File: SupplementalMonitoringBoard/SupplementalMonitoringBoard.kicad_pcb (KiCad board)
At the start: 2 copper layers, 53.5 x 77 mm, 47 parts, among them J1 PeripheralCANConnector, J2 PeripheralCANConnector, U1 OPA842xDBV, U2 OPA842xDBV, U3 INA180B1, U4 PAMC131M03QDFMRQ1, U5 PeripheralSOM

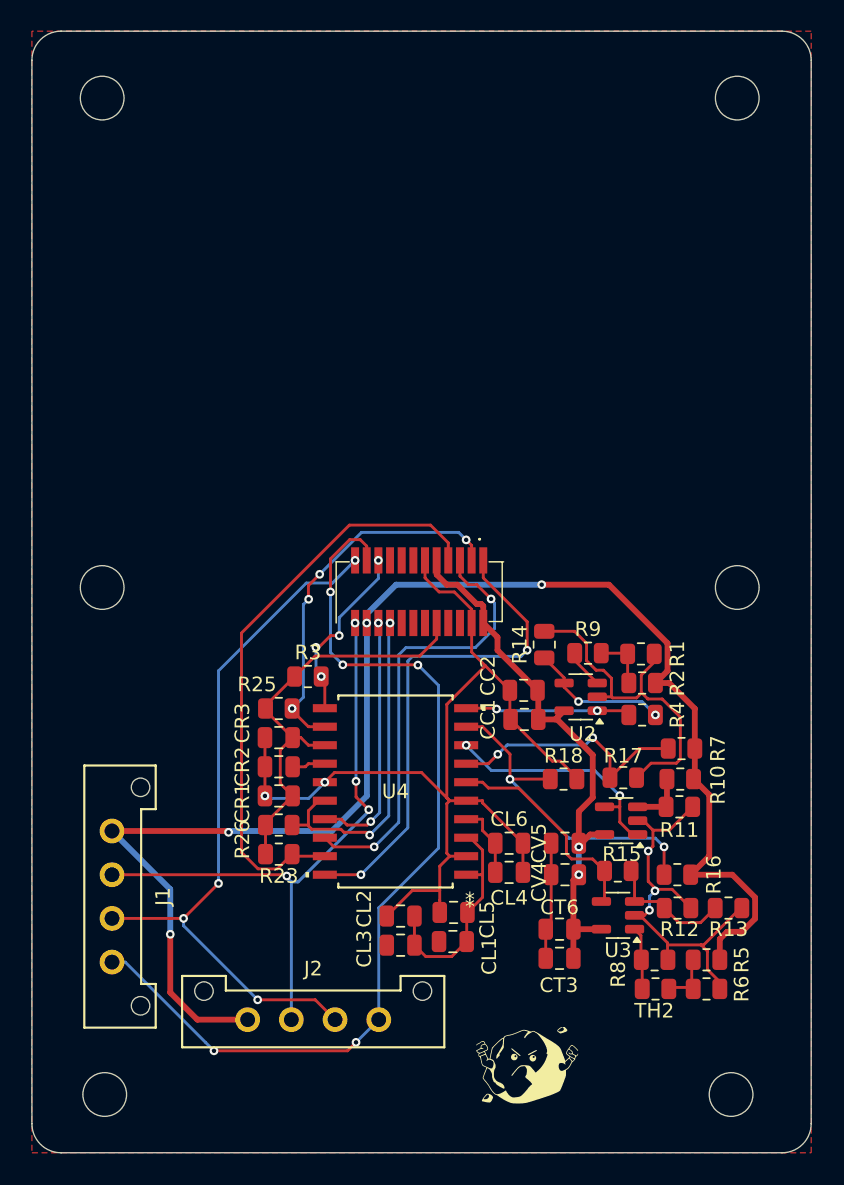
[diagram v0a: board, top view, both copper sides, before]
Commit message: Supplemental MOnitoring Board
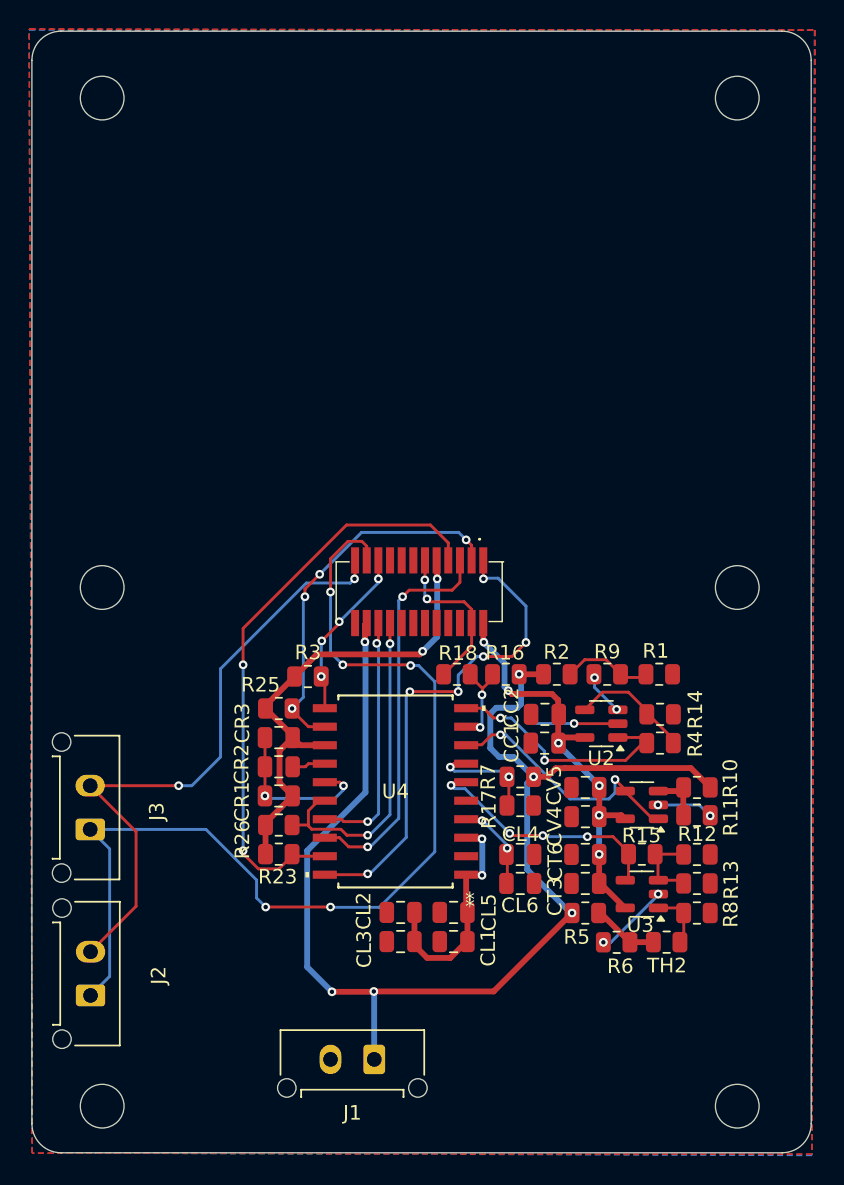
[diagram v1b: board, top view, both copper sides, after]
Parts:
- removed the ? at (124.5, 129.0)
- removed the ? at (167.5, 129.0)
- removed G***: LOGO, LOGO
- added ?: , , F.Cu at (167.9, 129.8)
- added ?: , , F.Cu at (124.3, 129.8)
- added J3: CANconn2, Connector_Molex:Molex_Micro-Fit_3.0_43650-0215_1x02_P3.00mm_Vertical, F.Cu at (123.5, 110.8)
- CC1, CT3, CV5: value .1uF -> 1nF
- CL2, CL5, CL6, CR1: value 1nF -> .1uF
- J1: value PeripheralCANConnector -> CarPowerConnector; footprint UTSVT_Connectors:Molex_MicroFit3.0_1x4xP3.00mm_PolarizingPeg_Vertical -> Connector_Molex:Molex_Micro-Fit_3.0_43650-0215_1x02_P3.00mm_Vertical
- J2: value PeripheralCANConnector -> CANconn; footprint UTSVT_Connectors:Molex_MicroFit3.0_1x4xP3.00mm_PolarizingPeg_Vertical -> Connector_Molex:Molex_Micro-Fit_3.0_43650-0215_1x02_P3.00mm_Vertical
- R14: value 150K -> 150k
- R2: value 50K -> 50k
- R4: value 10K -> 10k
- R7: value 30K -> 30k
- TH2: value 500 -> 500.
- moved J1 23.9 mm to (143.0, 126.6), turned to 180 degrees
- moved R16 18.1 mm to (152.0, 100.2)
- moved R7 11.2 mm to (153.0, 107.2)
- moved J2 10.9 mm to (123.5, 122.2), turned to 90 degrees
- moved R18 10.3 mm to (148.7, 100.2), turned to 180 degrees
- moved R14 9.28 mm to (162.6, 102.9), turned to 180 degrees
- moved R5 8.92 mm to (157.5, 116.5), turned to 180 degrees
- moved R17 7.32 mm to (153.0, 109.2)
- moved R6 6.95 mm to (159.6, 118.5), turned to 180 degrees
- moved R2 5.89 mm to (155.5, 100.2), turned to 180 degrees
- moved CT3 5.44 mm to (157.5, 114.5)
- moved CT6 5.43 mm to (157.5, 112.5)
- moved R8 4.33 mm to (165.2, 116.5)
- moved CV4 4.22 mm to (157.5, 109.9)
- moved CV5 4.08 mm to (157.5, 107.9)
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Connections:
- J1 pad 1: +BATT -> +12V
- J1 pad 2: GNDPWR -> GND
- J2 pad 1: +BATT -> /CAN_L
- J2 pad 2: GNDPWR -> /CAN_H
- R10 pad 2: +BATT -> +12V
- R16 pad 2: +BATT -> +12V
- R2 pad 2: +BATT -> +12V
- R5 pad 2: +BATT -> +12V
- R7 pad 2: +BATT -> +12V
- U5 pad 10: /DVDD -> unconnected-(U5-VDDA(3.3V)-Pad10)
- U5 pad 22: +BATT -> +12V
- U5 pad 9: +3.3V -> /DVDD
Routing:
- net +BATT: track 102.8 -> 0.00 mm, vias 4 -> 0
- net GND: track 131.7 -> 38.1 mm, vias 5 -> 9
- net +12V: track 0.00 -> 87.0 mm, vias 0 -> 6
- net GNDPWR: track 42.8 -> 0.00 mm, vias 4 -> 0
- net /AINOP: track 22.8 -> 5.97 mm
- net /AIN12N: track 17.5 -> 7.46 mm
- net +3.3V: track 38.4 -> 29.3 mm, vias 2 -> 6
- net /CAN_H: track 48.8 -> 42.9 mm, vias 4 -> 2
- net /AIN0N: track 11.4 -> 16.9 mm
- net /CAN_L: track 65.5 -> 70.9 mm
- net /DVDD: track 29.6 -> 33.8 mm, vias 0 -> 2
- net /SCLK: track 30.8 -> 27.3 mm
- net Net-(U3--): track 8.75 -> 5.66 mm
- net /AIN2P/GPO: track 14.9 -> 17.4 mm, vias 0 -> 4
- net Net-(R1-Pad1): track 3.87 -> 6.04 mm
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- added copper zone on B.Cu, net GND
